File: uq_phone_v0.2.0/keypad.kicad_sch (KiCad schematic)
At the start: 59 parts, among them SW1 SKTAAAE010, SW10 SKTAAAE010, SW11 SKTAAAE010, SW12 SKTAAAE010, SW13 SKTAAAE010, SW14 SKTAAAE010, SW15 SKTAAAE010, SW16 SKSCLCE010, SW17 SKTAAAE010, SW18 SKTAAAE010, SW19 SKTAAAE010, SW2 SKTAAAE010, SW20 SKTAAAE010, SW21 SKTAAAE010, SW22 SKSCLCE010, SW23 SKTAAAE010, SW24 SKTAAAE010, SW25 SKTAAAE010, SW26 SKTAAAE010, SW27 SKTAAAE010, SW28 SKTAAAE010, SW29 SKTAAAE010, SW3 SKTAAAE010, SW30 SKTAAAE010, SW31 SKTAAAE010, SW32 SKTAAAE010, SW33 SKTAAAE010, SW34 SKTAAAE010, SW35 SKTAAAE010, SW36 SKTAAAE010, SW37 SKTAAAE010, SW38 SKTAAAE010, SW39 SKTAAAE010, SW4 SKTAAAE010, SW40 SKTAAAE010, SW41 SKTAAAE010, SW5 SKTAAAE010, SW6 SKSCLCE010, SW7 SKTAAAE010, SW8 SKTAAAE010, SW9 SKTAAAE010

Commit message: Routing Update
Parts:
- LED2: now left out of the parts list
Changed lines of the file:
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@@
 		(unit 1)
 		(exclude_from_sim no)
-		(in_bom yes)
+		(in_bom no)
 		(on_board yes)
 		(dnp no)

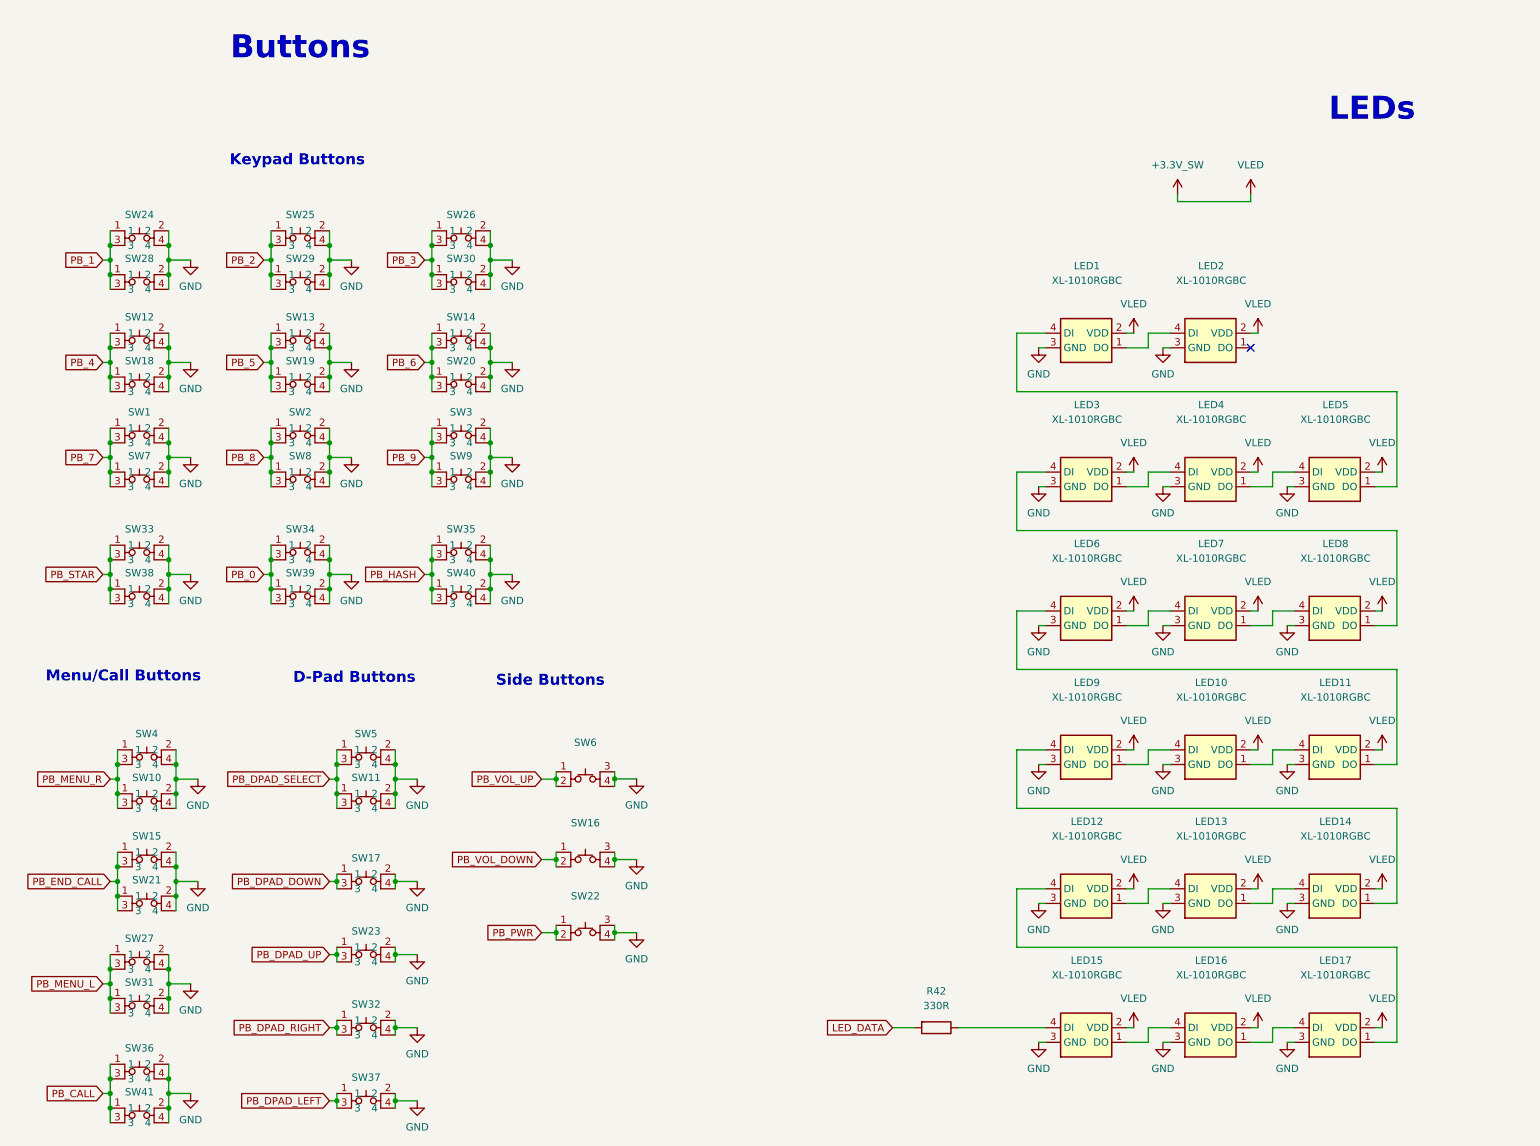
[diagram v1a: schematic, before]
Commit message: Cleaning up adn fixing massive mistake
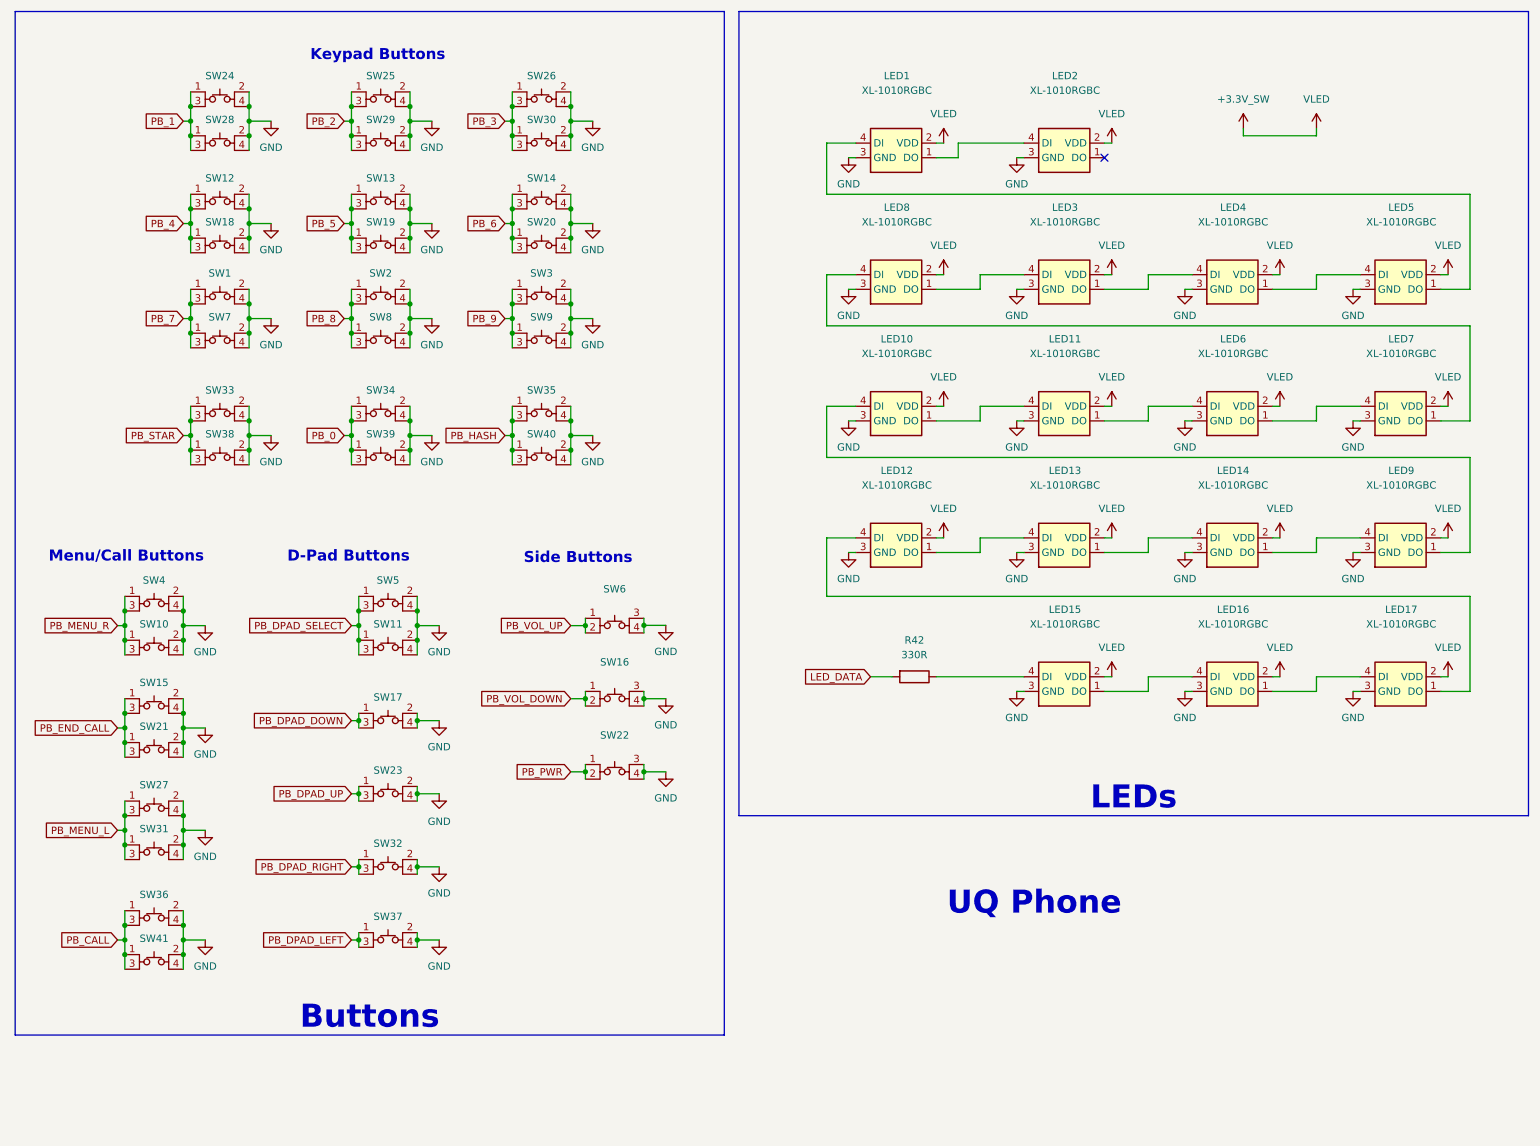
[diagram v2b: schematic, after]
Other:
- note added: "UQ Phone"
- note removed: "Buttons"
- note removed: "LEDs"
- title: UQ Phone -> Keypad
- moved on the sheet: LED1, LED10, LED11, LED12, LED13, LED14, LED15, LED16, LED17, LED2, LED3, LED4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
